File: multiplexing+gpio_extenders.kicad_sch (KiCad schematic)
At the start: 3 parts, among them IC4 PEC12R-4230F-S0024, U12 CD4052B, U13 CD4052B

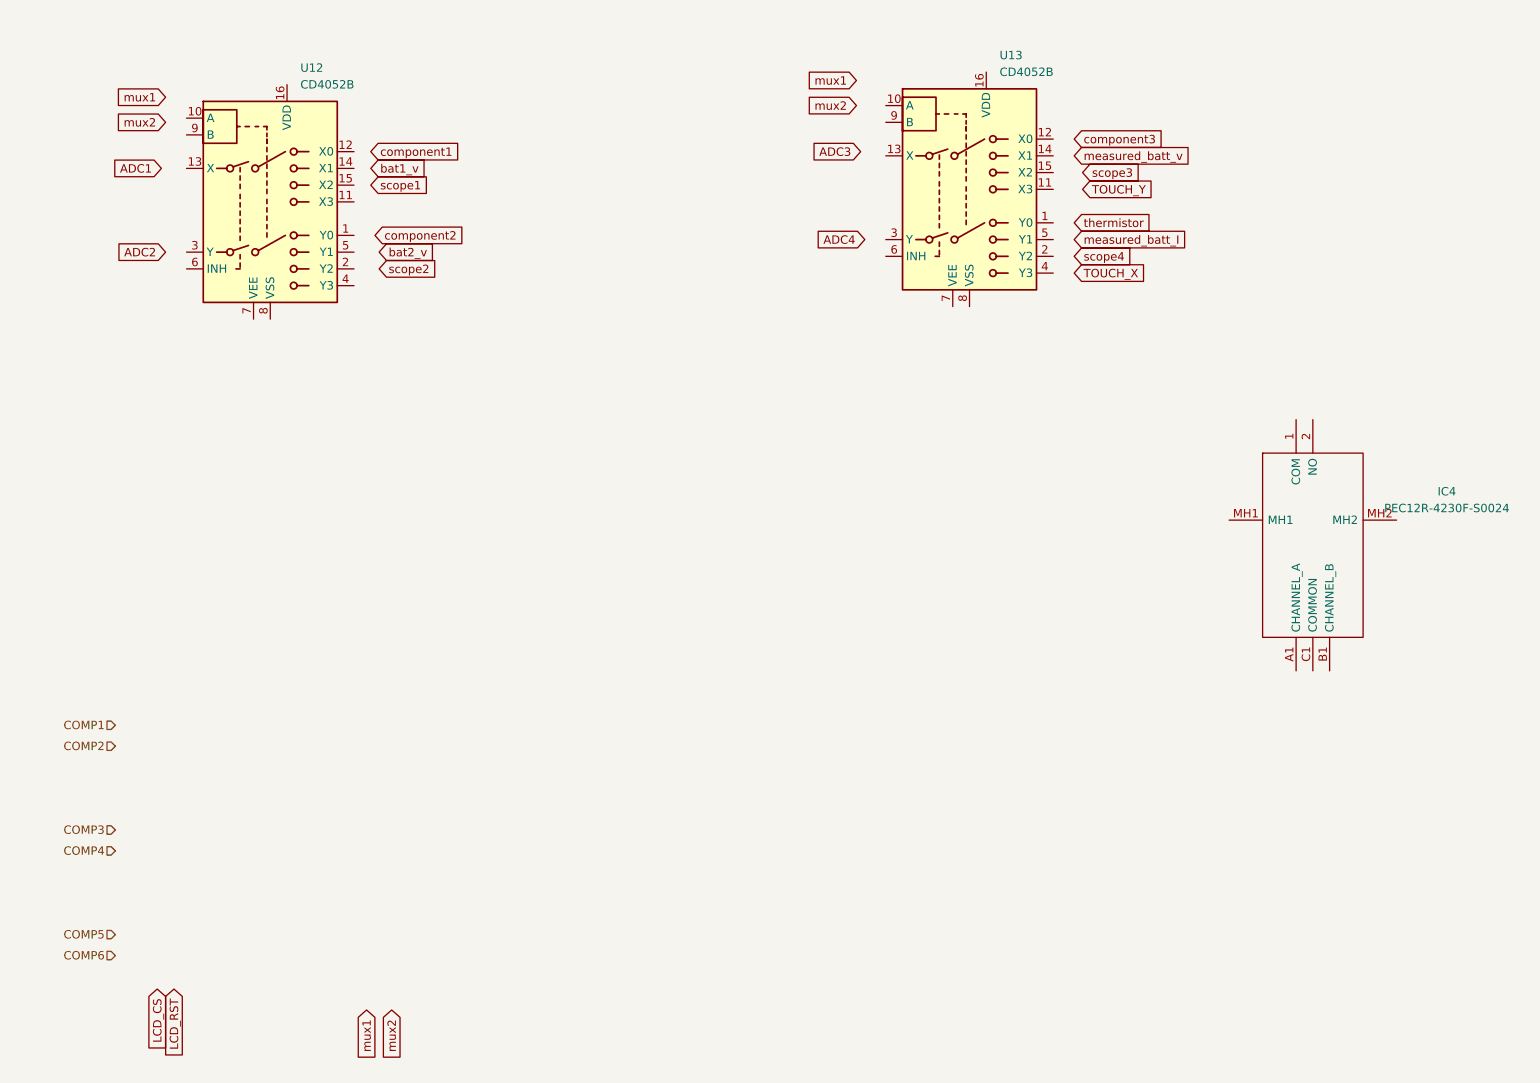
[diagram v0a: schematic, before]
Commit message: h
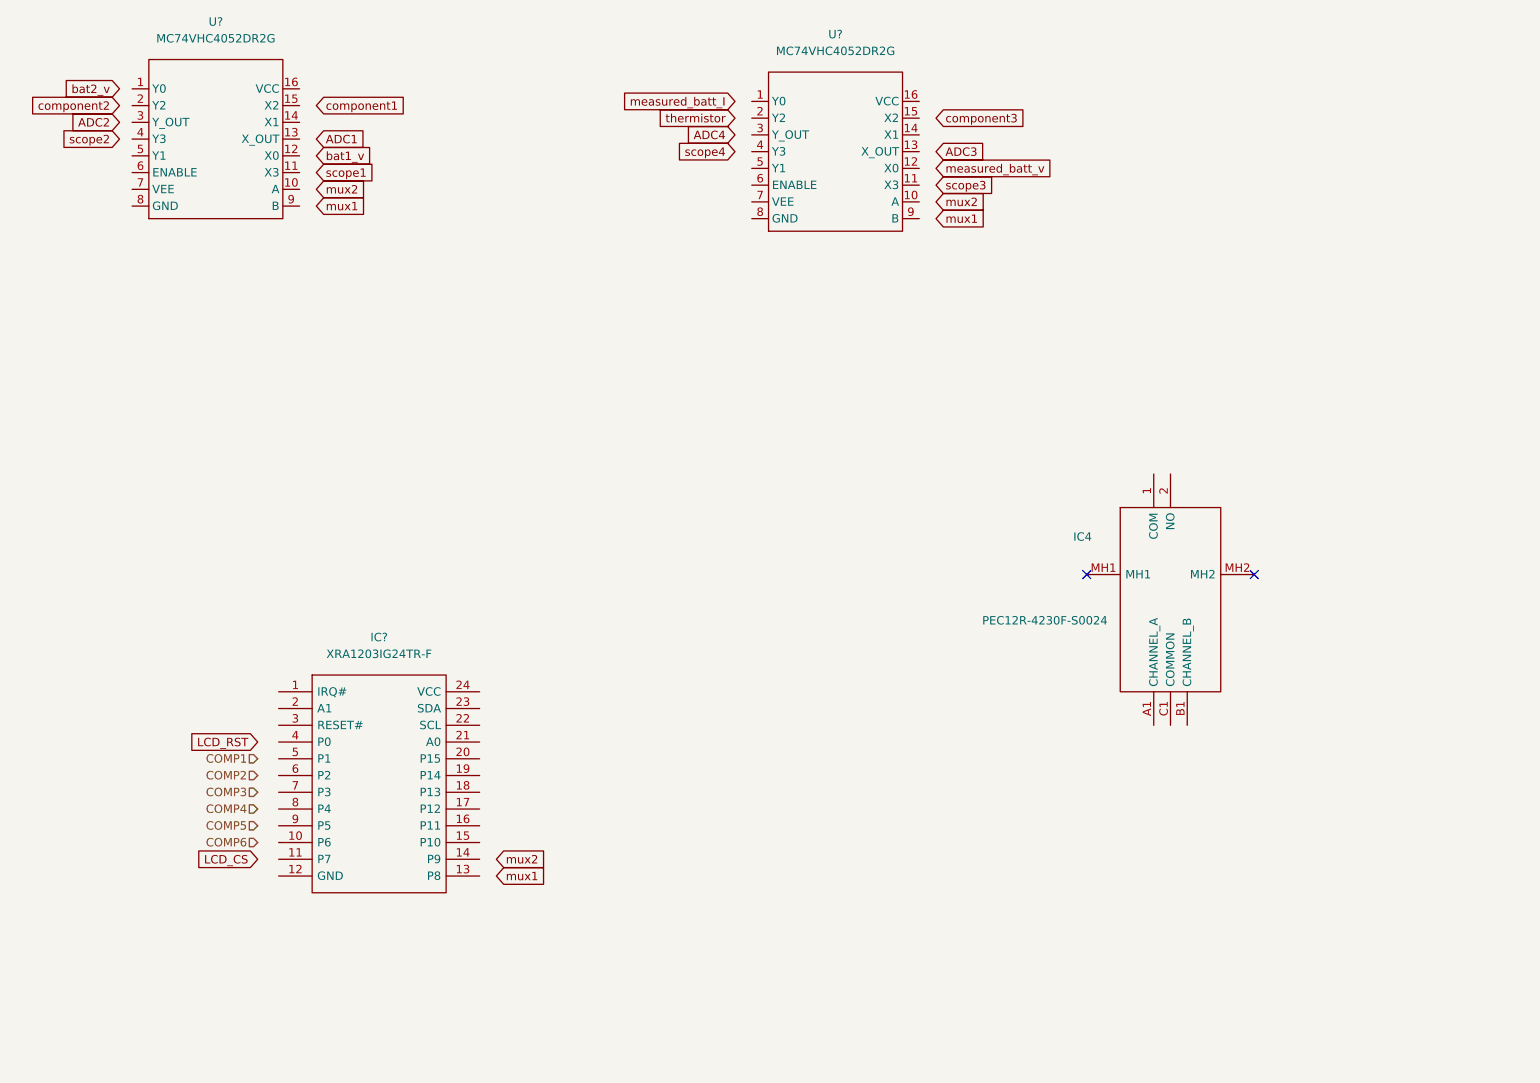
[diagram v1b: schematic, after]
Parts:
- removed U12, U13: CD4052B, symbol Analog_Switch:CD4052B
- added IC?: XRA1203IG24TR-F, SOP65P640X120-24N, symbol SamacSys_Parts:XRA1203IG24TR-F
- added U? (x2): MC74VHC4052DR2G, Package_SO:SOIC-16_3.9x9.9mm_P1.27mm, symbol My_custom_lib:MC74VHC4052DR2G
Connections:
- no-connect marks 0 -> 2
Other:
- moved on the sheet: IC4
